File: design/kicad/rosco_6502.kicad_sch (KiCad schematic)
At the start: 56 parts, among them IC1 W65C02SxP, IC2 ATF22V10C-7PX, IC3 XR68C681CJTR-F, IC4 NE555P, IC5 ATF22V10C-7PX, J1 UART_A, J2 UART_B, J3 Conn_01x06, J4 Conn_01x01_Male, J5 Conn_02x18_Odd_Even, J6 Conn_01x02_Male, J7 Jack-DC, Q1 3.6864MHz, U1 AS6C4008-55PCN, U2 AS6C62256-55PCN, U3 AT28C64B-15PU, U4 74HCT174, X1 14MHz

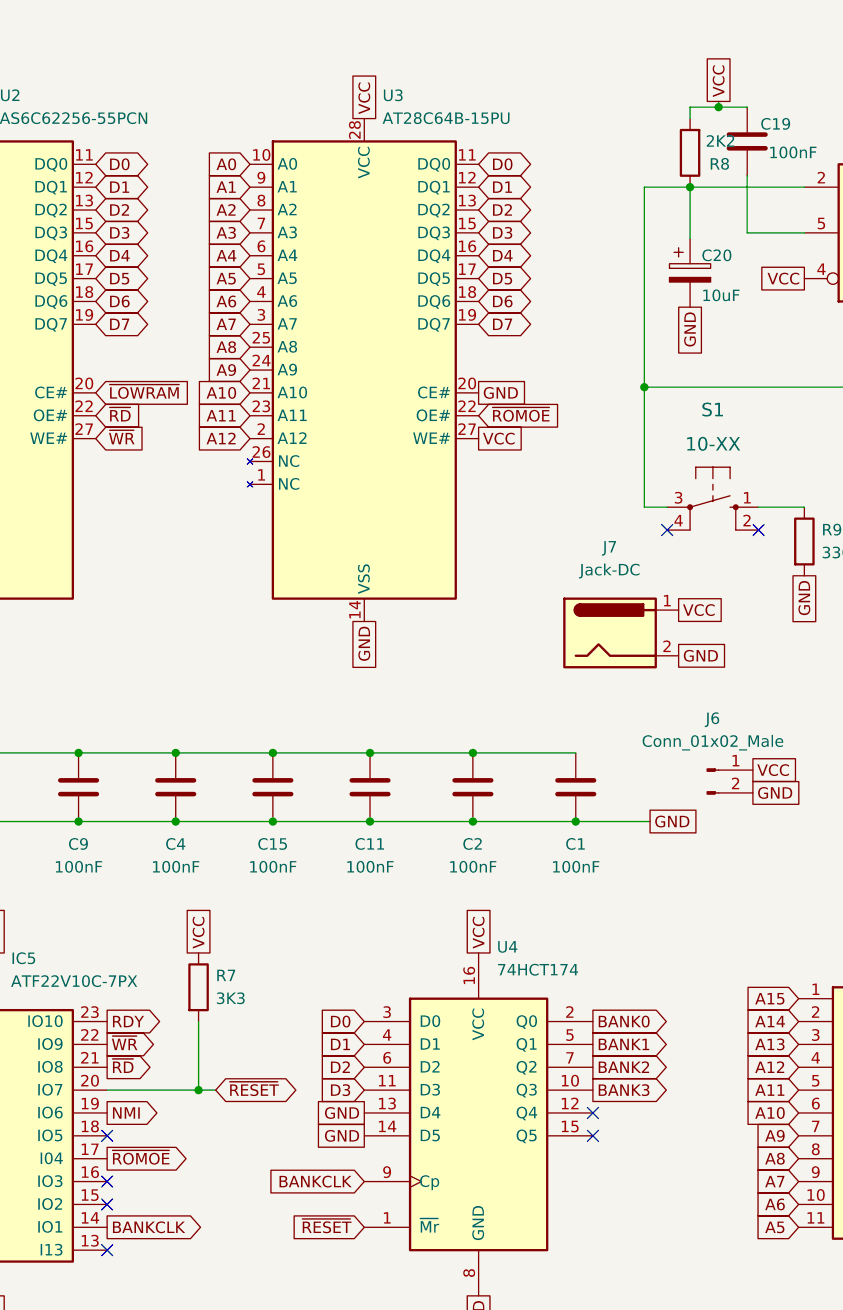
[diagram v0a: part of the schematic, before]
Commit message: Bank ROM
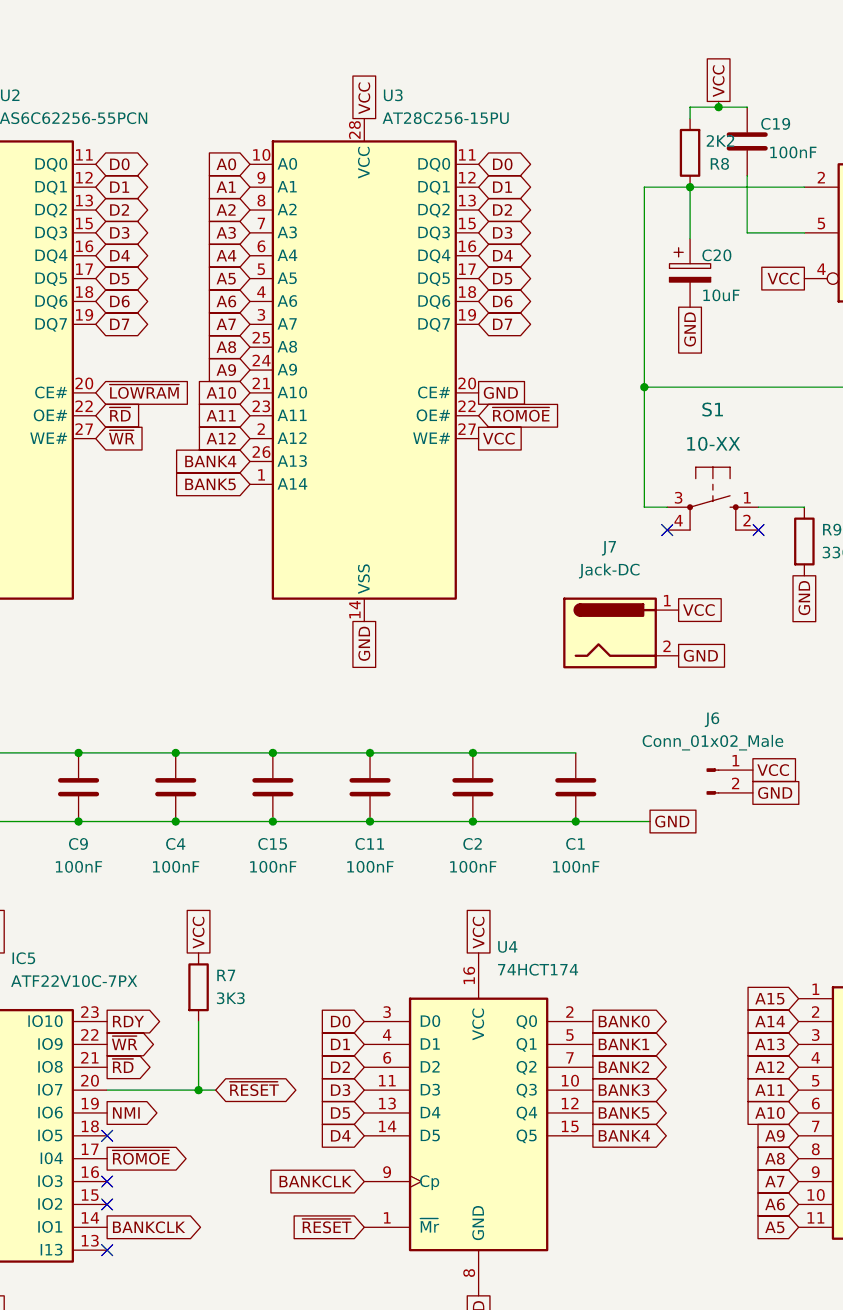
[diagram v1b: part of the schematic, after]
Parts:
- U3: value AT28C64B-15PU -> AT28C256-15PU; footprint Package_DIP:DIP-28_W15.24mm_Socket_LongPads -> Package_DIP:DIP-28_W15.24mm; symbol rosco_6502:AT28C64B -> rosco_6502:AT28C256
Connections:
- net D4: now also U4.14 (D5)
- net D5: now also U4.13 (D4)
- net GND: no longer U4.13 (D4), U4.14 (D5)
- net BANK5: now reaches U3.1 (A14)
- net BANK5: now also U4.12 (Q4)
- net BANK4: now reaches U3.26 (A13)
- net BANK4: now also U4.15 (Q5)
- no-connect marks 13 -> 11
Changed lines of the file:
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@@
   (title_block
     (title "rosco_6502")
-    (date "2022-07-16")
+    (date "2023-09-10")
     (rev "3")
     (company "The Really Old-School Company Limited")
-    (comment 1 "Copyright (c)2022 Ross Bamford & Contributors")
+    (comment 1 "Copyright (c)2022-2023 Ross Bamford & Contributors")
     (comment 2 "Open Source Hardware (CERN OHL)")
   )
@@
   (no_connect (at 106.68 125.095))
   (no_connect (at 106.68 122.555))
-  (no_connect (at 220.345 132.715))
-  (no_connect (at 220.345 135.255))
   (no_connect (at 166.37 142.875))
   (no_connect (at 166.37 147.955))
@@
     (effects (font (size 1.27 1.27)) (justify left bottom))
   )
+  (global_label "BANK5" (shape output) (at 220.345 132.715 0) (fields_autoplaced)
+    (effects (font (size 1.27 1.27)) (justify left))
+    (property "Intersheet References" "${INTERSHEET_REFS}" (id 0) (at 228.9267 132.6356 0)
+      (effects (font (size 1.27 1.27)) (justify left) hide)
+    )
+  )
   (global_label "VCC" (shape passive) (at 45.085 120.015 90) (fields_autoplaced)
     (effects (font (size 1.27 1.27)) (justify left))
@@
     )
   )
-  (global_label "GND" (shape passive) (at 194.945 135.255 180) (fields_autoplaced)
+  (global_label "D5" (shape input) (at 194.945 132.715 180) (fields_autoplaced)
     (effects (font (size 1.27 1.27)) (justify right))
-    (property "Intersheet References" "${INTERSHEET_REFS}" (id 0) (at 188.6614 135.1756 0)
+    (property "Intersheet References" "${INTERSHEET_REFS}" (id 0) (at 190.0524 132.6356 0)
       (effects (font (size 1.27 1.27)) (justify right) hide)
     )
@@
     )
   )
-  (global_label "GND" (shape passive) (at 194.945 132.715 180) (fields_autoplaced)
+  (global_label "D4" (shape input) (at 194.945 135.255 180) (fields_autoplaced)
     (effects (font (size 1.27 1.27)) (justify right))
-    (property "Intersheet References" "${INTERSHEET_REFS}" (id 0) (at 188.6614 132.6356 0)
+    (property "Intersheet References" "${INTERSHEET_REFS}" (id 0) (at 190.0524 135.1756 0)
       (effects (font (size 1.27 1.27)) (justify right) hide)
     )
@@
     )
   )
+  (global_label "BANK4" (shape output) (at 220.345 135.255 0) (fields_autoplaced)
+    (effects (font (size 1.27 1.27)) (justify left))
+    (property "Intersheet References" "${INTERSHEET_REFS}" (id 0) (at 228.9267 135.1756 0)
+      (effects (font (size 1.27 1.27)) (justify left) hide)
+    )
+  )
   (global_label "A5" (shape input) (at 256.54 74.93 180) (fields_autoplaced)
     (effects (font (size 1.27 1.27)) (justify right))
@@
     )
   )
+  (global_label "BANK4" (shape input) (at 182.245 60.325 180) (fields_autoplaced)
+    (effects (font (size 1.27 1.27)) (justify right))
+    (property "Intersheet References" "${INTERSHEET_REFS}" (id 0) (at 173.6633 60.2456 0)
+      (effects (font (size 1.27 1.27)) (justify right) hide)
+    )
+  )
   (global_label "A7" (shape input) (at 182.245 45.085 180) (fields_autoplaced)
     (effects (font (size 1.27 1.27)) (justify right))
@@
     )
   )
+  (global_label "BANK5" (shape input) (at 182.245 62.865 180) (fields_autoplaced)
+    (effects (font (size 1.27 1.27)) (justify right))
+    (property "Intersheet References" "${INTERSHEET_REFS}" (id 0) (at 173.6633 62.7856 0)
+      (effects (font (size 1.27 1.27)) (justify right) hide)
+    )
+  )
   (global_label "VCC" (shape passive) (at 176.53 114.935 90) (fields_autoplaced)
     (effects (font (size 1.27 1.27)) (justify left))
@@
     (pin "2")
   )
-  (symbol (lib_id "rosco_6502:AT28C64B") (at 194.945 50.165 0) (unit 1)
+  (symbol (lib_id "rosco_6502:AT28C256") (at 194.945 50.165 0) (unit 1)
     (in_bom yes) (on_board yes) (fields_autoplaced)
     (property "Reference" "U3" (id 0) (at 196.9644 19.685 0)
       (effects (font (size 1.27 1.27)) (justify left))
     )
-    (property "Value" "AT28C64B-15PU" (id 1) (at 196.9644 22.225 0)
+    (property "Value" "AT28C256-15PU" (id 1) (at 196.9644 22.225 0)
       (effects (font (size 1.27 1.27)) (justify left))
     )
-    (property "Footprint" "Package_DIP:DIP-28_W15.24mm_Socket_LongPads" (id 2) (at 194.945 92.075 0)
+    (property "Footprint" "Package_DIP:DIP-28_W15.24mm" (id 2) (at 194.945 92.075 0)
       (effects (font (size 1.27 1.27)) hide)
     )
-    (property "Datasheet" "https://ww1.microchip.com/downloads/aemDocuments/documents/MPD/ProductDocuments/DataSheets/AT28C64B-64K-%288Kx8%29-Industrial-Parallel-EEPROM-with-Page-Write-and-Software-Data-Protection-20006432A.pdf" (id 3) (at 194.945 89.535 0)
+    (property "Datasheet" "https://ww1.microchip.com/downloads/en/DeviceDoc/doc0006.pdf" (id 3) (at 194.945 89.535 0)
       (effects (font (size 1.27 1.27)) hide)
     )
@@
     )
     (path "/4538bf2d-4cfd-4cc4-8255-e988871e9c9f"
-      (reference "U3") (unit 1) (value "AT28C64B-15PU") (footprint "Package_DIP:DIP-28_W15.24mm_Socket_LongPads")
+      (reference "U3") (unit 1) (value "AT28C256-15PU") (footprint "Package_DIP:DIP-28_W15.24mm")
     )
     (path "/7935fa25-e96e-4855-a3e0-7a704a6c1626"
